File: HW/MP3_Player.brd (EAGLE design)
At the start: 210 x 15 mm, 81 parts, among them J1 Audio jack, J2 LIPO-BATTERY-CONNECTOR, J3 USD-SDIO-SOCKETJLH, J4 micro USB, Q1 8MHz, Q2 12.288MHz, U1 3.3V/150mA, U2 1.8V/100mA, U3 ATMEGA32U4QFN, U4 VS1053B, U5 MCP73831

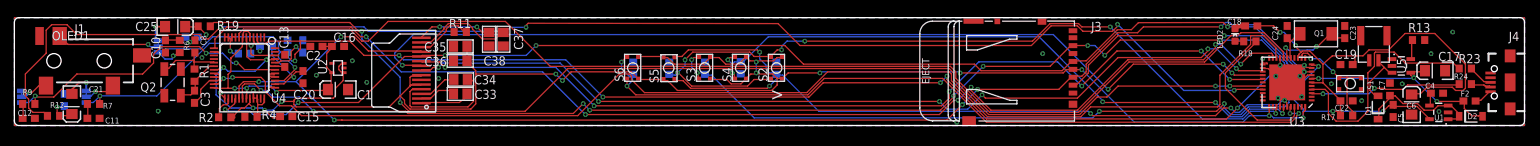
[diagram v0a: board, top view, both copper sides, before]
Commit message: atmega routed
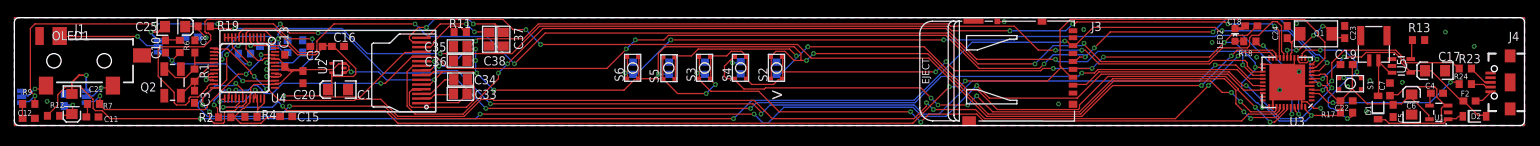
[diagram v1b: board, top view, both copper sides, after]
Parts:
- moved D2 0.50 mm to (203.0, 1.28)
- moved R17 0.40 mm to (185.3, 1.80)
- moved C11 0.25 mm to (10.8, 1.20)
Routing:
- net 3.3V: track 362.8 -> 294.2 mm, vias 20 -> 21
- net GBUF: track 41.7 -> 64.1 mm, vias 3 -> 5
- net MP3-CS: track 169.1 -> 185.7 mm, vias 2 -> 4
- net GND: track 16.1 -> 31.2 mm
- net MOSI: track 183.3 -> 198.4 mm, vias 7 -> 5
- net 1.8V: track 36.7 -> 50.6 mm, vias 3 -> 5
- net PWM_L: track 194.3 -> 181.2 mm
- net MISO: track 164.1 -> 175.9 mm, vias 10 -> 6
- net RIGHT: track 30.8 -> 19.7 mm
- net VIN: track 17.2 -> 26.1 mm
- net RST: track 16.1 -> 24.1 mm, vias 2 -> 4
- net N$1: track 21.9 -> 14.1 mm, vias 0 -> 2
- net N$22: track 33.2 -> 25.7 mm, vias 0 -> 2
- net PWM_R: track 161.7 -> 154.8 mm, vias 4 -> 6
- net SD-CS: track 39.4 -> 45.4 mm
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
